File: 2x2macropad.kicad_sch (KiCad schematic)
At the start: 14 parts, among them SW1 SW_Push, U1 ATmega32U4-A, Y1 16MHz

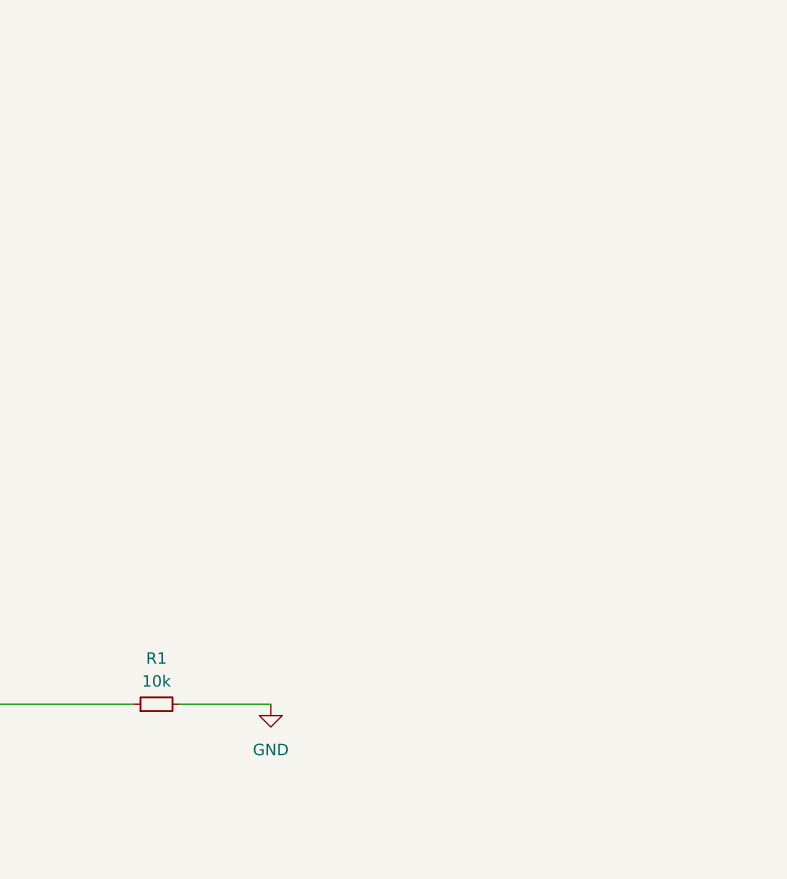
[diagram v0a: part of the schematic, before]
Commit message: Update kicad file
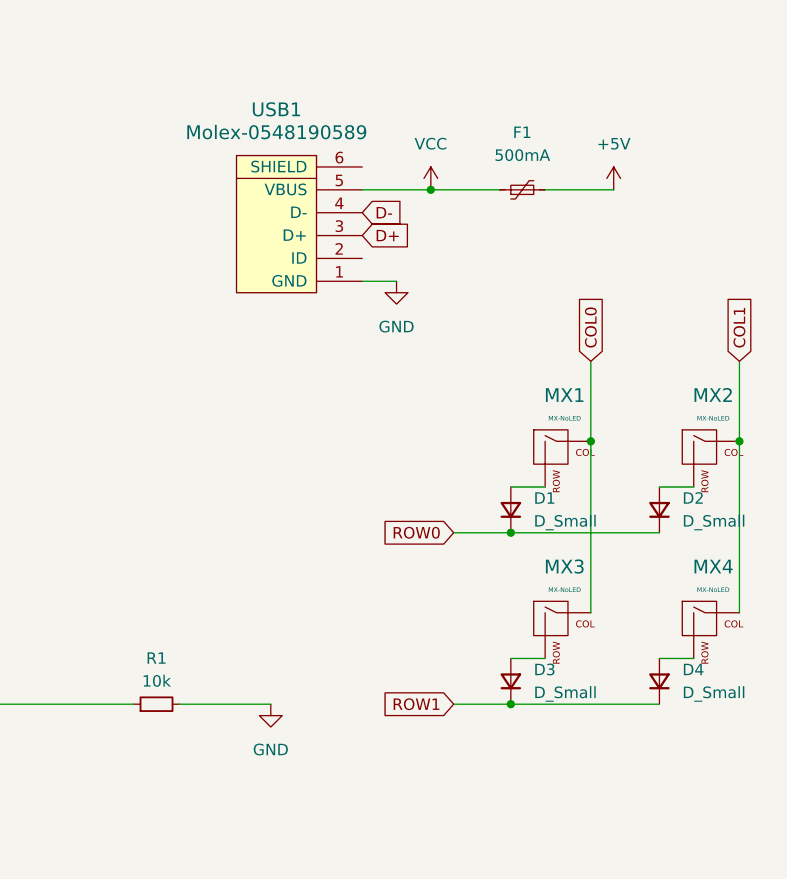
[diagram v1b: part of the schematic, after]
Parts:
- added D1, D2, D3, D4: D_Small, symbol Device:D_Small
- added F1: 500mA, symbol Device:Polyfuse_Small
- added MX1, MX2, MX3, MX4: MX-NoLED, symbol MX_Alps_Hybrid:MX-NoLED
- added USB1: Molex-0548190589, symbol random-keyboard-parts:Molex-0548190589
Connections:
- net +5V: now also F1.2
- net D+: now also USB1.3 (D+)
- net D-: now also USB1.4 (D-)
- net GND: now also USB1.1 (GND)
- new net: D2.2 (A), MX2.2 (ROW)
- new net: D4.2 (A), MX4.2 (ROW)
- new net: D1.2 (A), MX1.2 (ROW)
- new net: D3.2 (A), MX3.2 (ROW)
- new net COL0: MX1.1 (COL), MX3.1 (COL)
- new net COL1: MX2.1 (COL), MX4.1 (COL)
- new net ROW0: D1.1 (K), D2.1 (K)
- new net ROW1: D3.1 (K), D4.1 (K)
- new net VCC: F1.1, USB1.5 (VBUS)
